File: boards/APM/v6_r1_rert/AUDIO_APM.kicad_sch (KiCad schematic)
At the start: 21 parts, among them J11 DAC_L_PRB, J12 Conn_01x02, J19 AudioPlug3, J23 VOL_L_CTRL, J24 VOL_R_CTRL, J7 DAC_R_PRB, U2 OPA1678

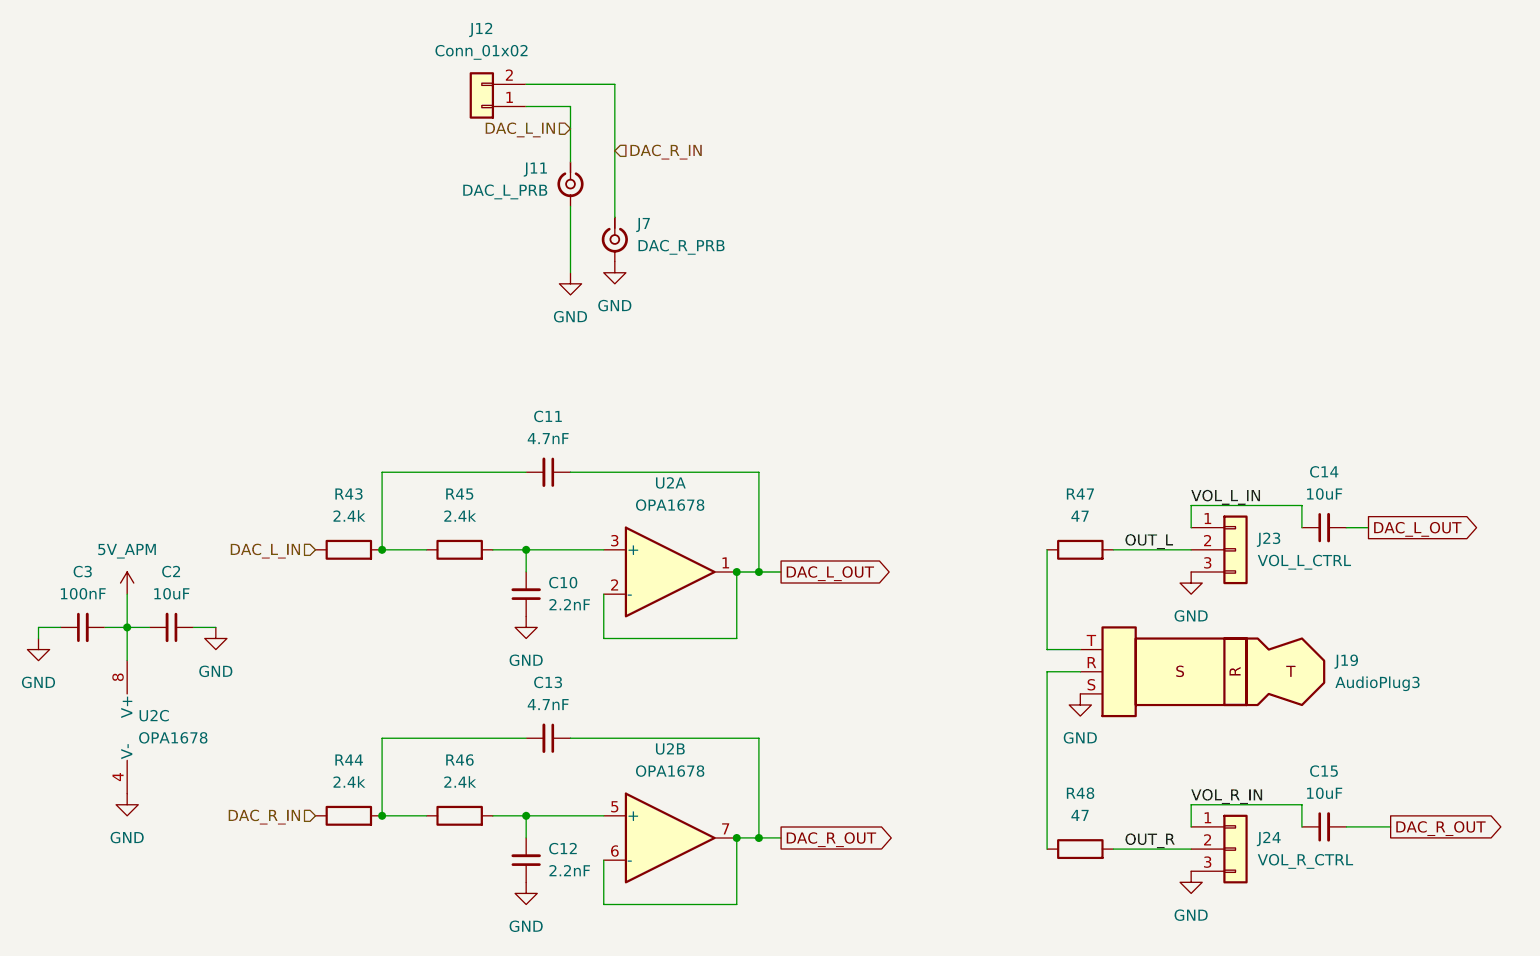
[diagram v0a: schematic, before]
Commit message: hmmm if i'm creating a minimal combination board maybe i don't blow up routing right now...
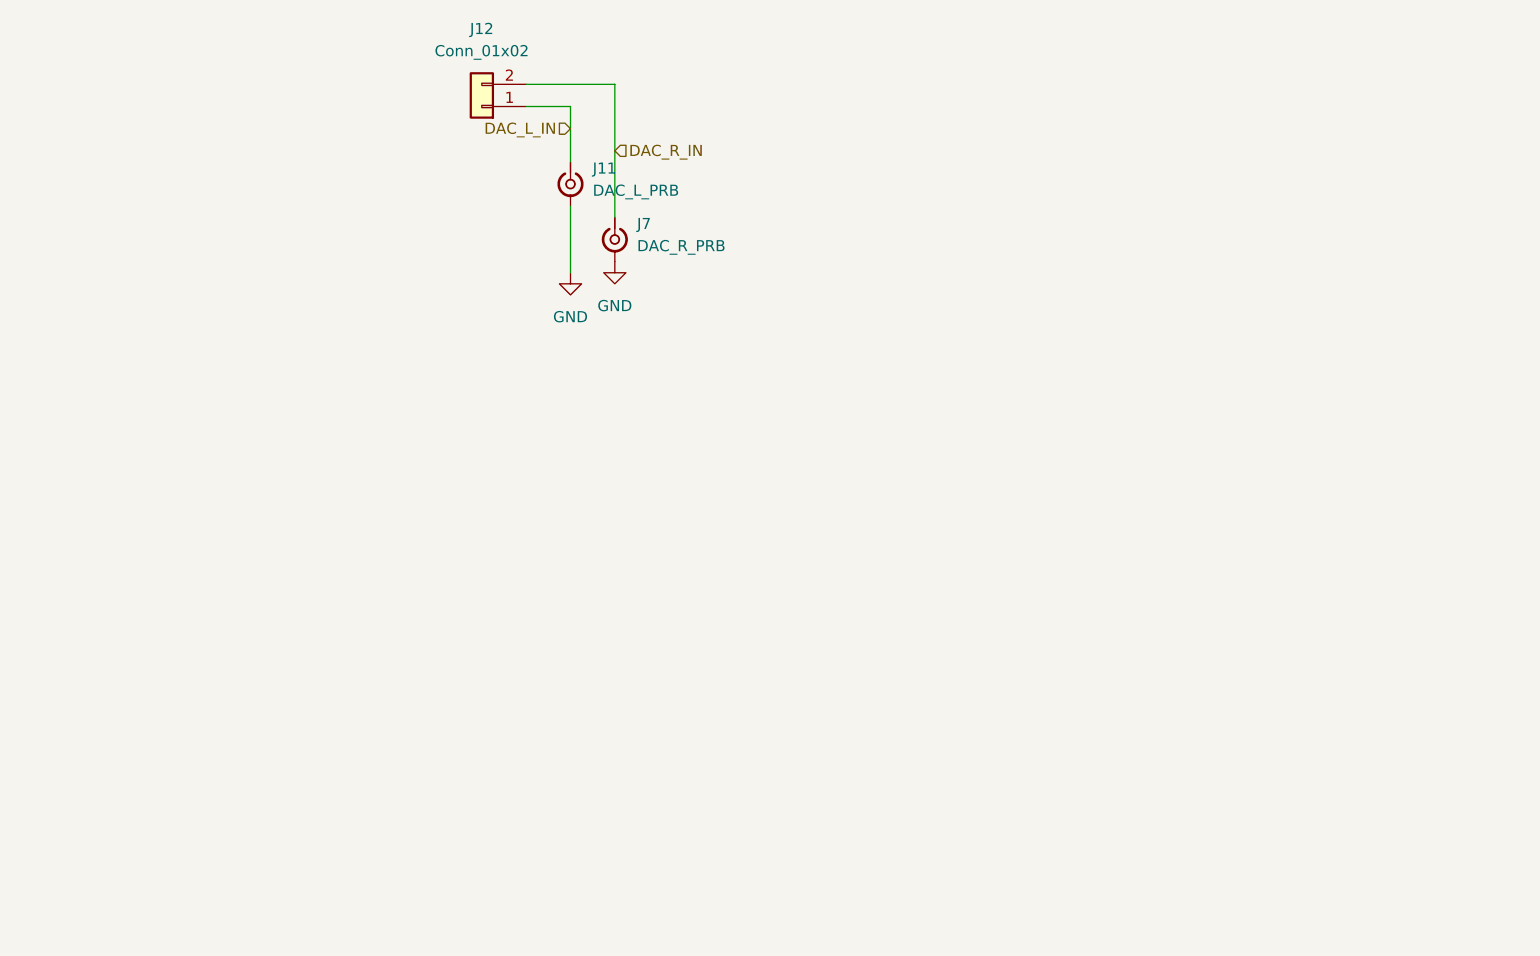
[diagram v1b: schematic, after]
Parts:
- removed C10, C12: 2.2nF, Capacitor_SMD:C_0805_2012Metric, symbol Device:C_Small
- removed C11, C13: 4.7nF, Capacitor_SMD:C_0805_2012Metric, symbol Device:C_Small
- removed C14, C15, C2: 10uF, Capacitor_SMD:CP_Elec_4x3, symbol Device:C_Small
- removed C3: 100nF, Capacitor_SMD:C_0805_2012Metric, symbol Device:C_Small
- removed J19: AudioPlug3, Connector_Audio:Jack_3.5mm_Ledino_KB3SPRS_Horizontal, symbol Connector_Audio:AudioPlug3
- removed J23: VOL_L_CTRL, Connector_PinHeader_2.54mm:PinHeader_1x03_P2.54mm_Vertical, symbol Connector_Generic:Conn_01x03
- removed J24: VOL_R_CTRL, Connector_PinHeader_2.54mm:PinHeader_1x03_P2.54mm_Vertical, symbol Connector_Generic:Conn_01x03
- removed R43, R44, R45, R46: 2.4k, Resistor_SMD:R_0201_0603Metric, symbol Device:R
- removed R47, R48: 47, Resistor_SMD:R_0201_0603Metric, symbol Device:R
- removed U2: OPA1678, Package_DIP:DIP-8_W7.62mm_SMDSocket_SmallPads, symbol Amplifier_Operational:OPA1678
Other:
- moved on the sheet: J11
